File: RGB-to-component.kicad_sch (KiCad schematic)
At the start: 58 parts, among them J1 VGA, J3 USB_C_Receptacle_Power, J4 SCART_CONN, J5 3xRCA_CONN, U1 SC6206B-65K5, U10 74HC86, U3 RS8752XK, U6 THS7374, U8 LM1881

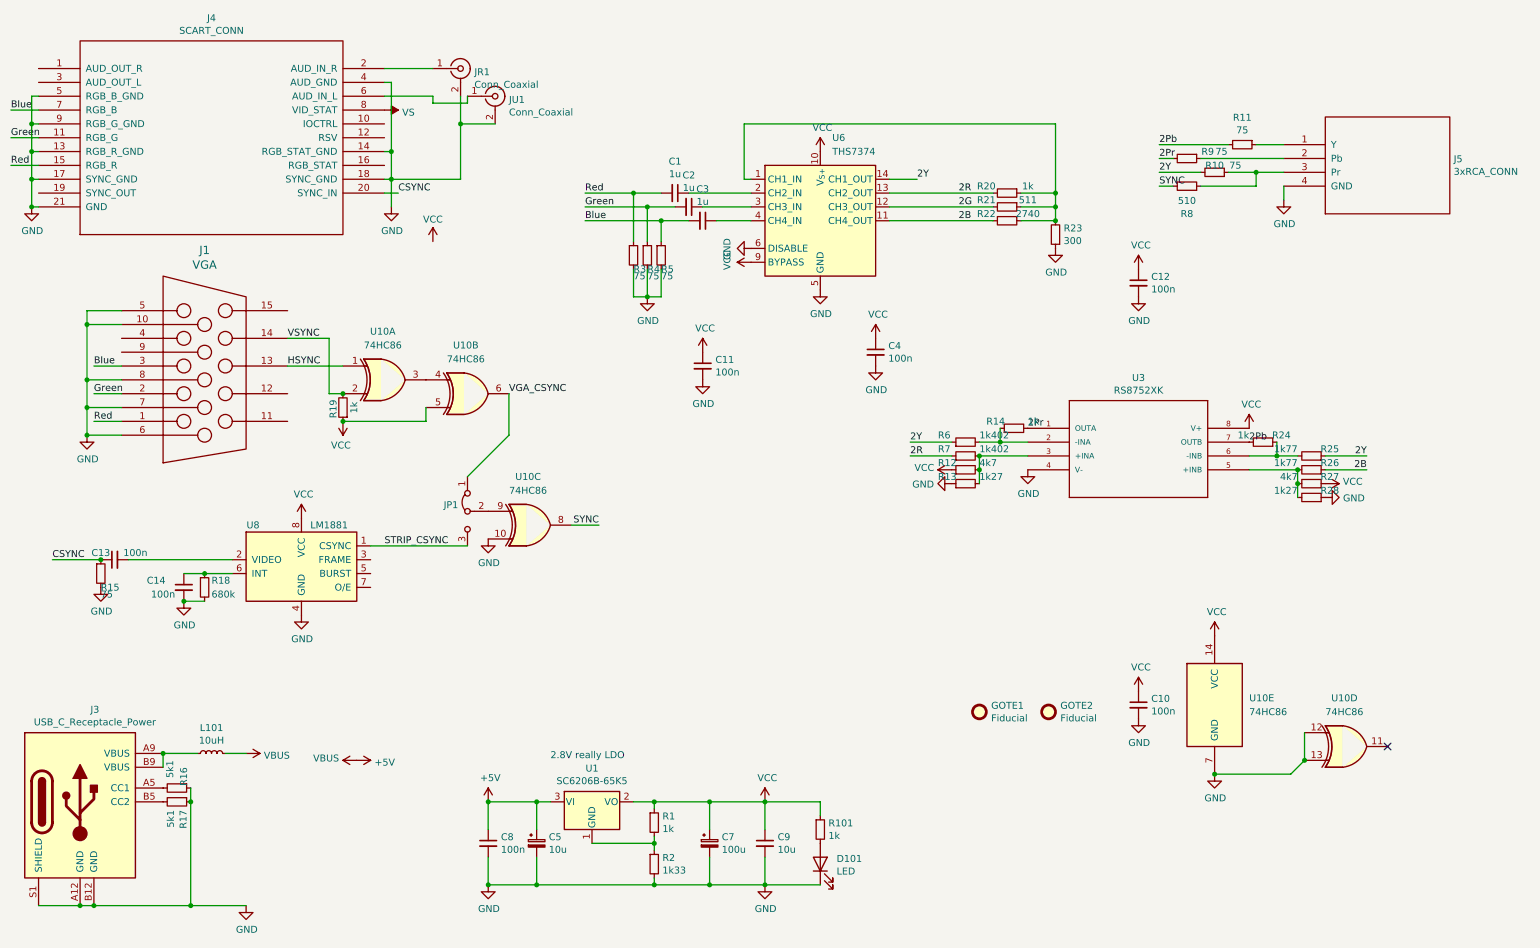
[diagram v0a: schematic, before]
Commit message: updated prod files
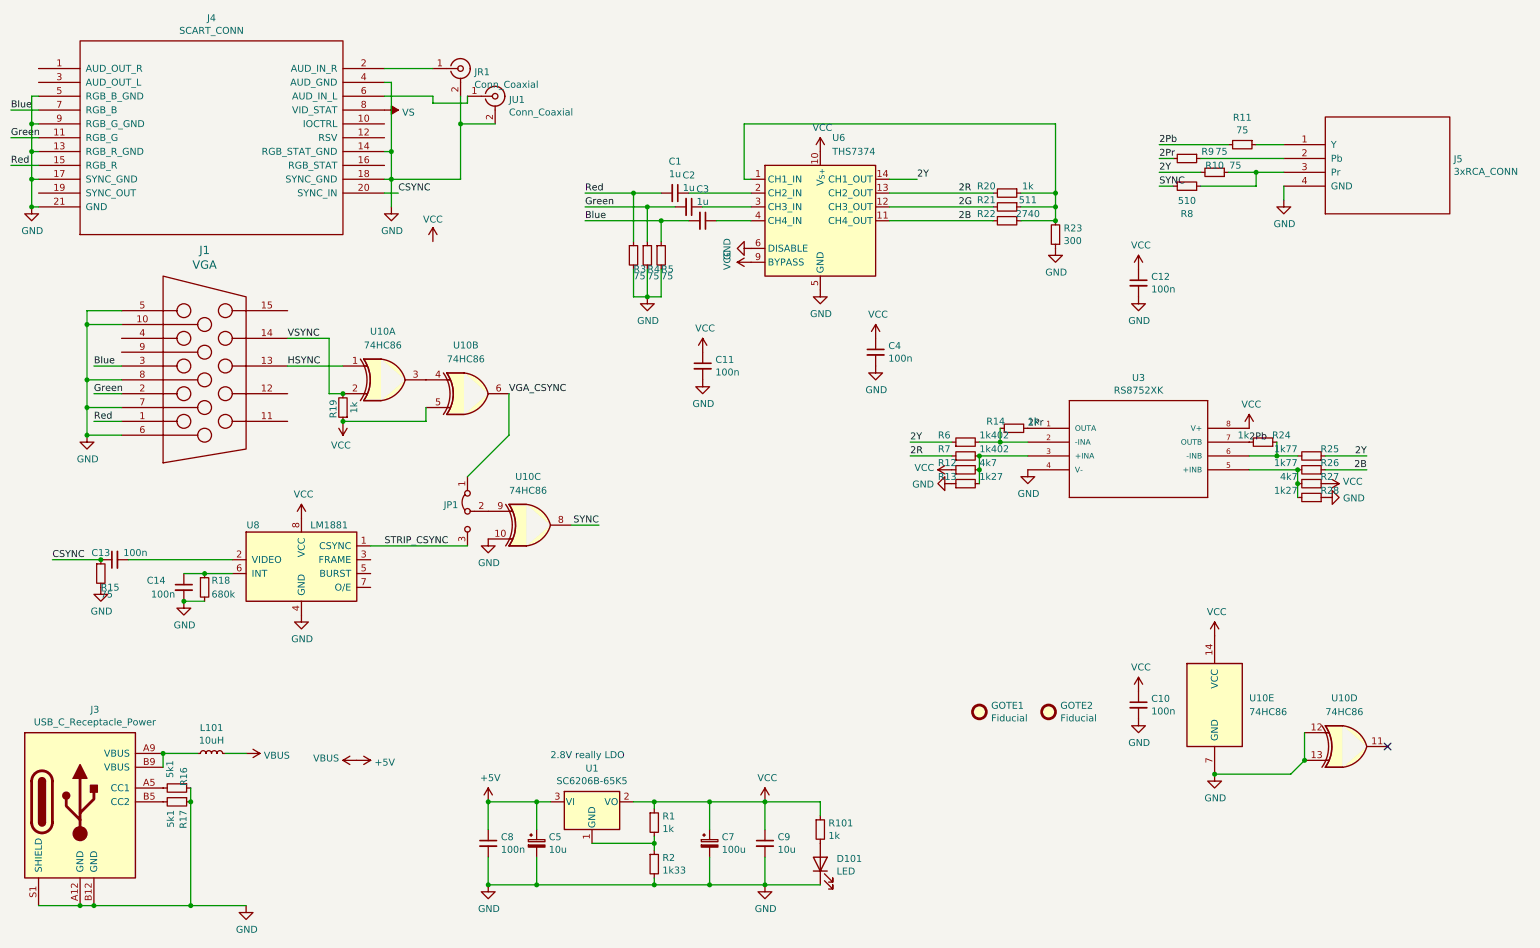
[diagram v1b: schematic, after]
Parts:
- U1: LCSC C130827 -> C2688243
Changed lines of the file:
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@@
 (kicad_sch
-	(version 20231120)
+	(version 20250114)
 	(generator "eeschema")
-	(generator_version "8.0")
+	(generator_version "9.0")
 	(paper "A4")
 	(title_block
@@
 		(comment 1 "KiCad gaming")
 	)
+	(text "2.8V really LDO"
+		(exclude_from_sim no)
+		(at 114.3 152.4 0)
+		(effects
+			(font
+				(size 1.27 1.27)
+			)
+			(justify left bottom)
+		)
+	)
 	(junction
 		(at 193.04 96.52)
@@
 		)
 	)
-	(text "2.8V really LDO"
-		(exclude_from_sim no)
-		(at 114.3 152.4 0)
-		(effects
-			(font
-				(size 1.27 1.27)
-			)
-			(justify left bottom)
-		)
-	)
 	(label "VGA_CSYNC"
 		(at 106.68 85.09 0)
-		(fields_autoplaced yes)
 		(effects
 			(font
@@
 	(label "2B"
 		(at 264.16 99.06 180)
-		(fields_autoplaced yes)
 		(effects
 			(font
@@
 	(label "Green"
 		(at 30.48 85.09 0)
-		(fields_autoplaced yes)
 		(effects
 			(font
@@
 	(label "Blue"
 		(at 120.65 53.34 0)
-		(fields_autoplaced yes)
 		(effects
 			(font
@@
 	(label "2Pb"
 		(at 242.57 93.98 0)
-		(fields_autoplaced yes)
 		(effects
 			(font
@@
 	(label "2Y"
 		(at 180.34 93.98 0)
-		(fields_autoplaced yes)
 		(effects
 			(font
@@
 	(label "Blue"
 		(at 15.24 33.02 0)
-		(fields_autoplaced yes)
 		(effects
 			(font
@@
 	(label "Green"
 		(at 120.65 50.8 0)
-		(fields_autoplaced yes)
 		(effects
 			(font
@@
 	(label "2G"
 		(at 189.23 50.8 0)
-		(fields_autoplaced yes)
 		(effects
 			(font
@@
 	(label "VSYNC"
 		(at 66.04 74.93 0)
-		(fields_autoplaced yes)
 		(effects
 			(font
@@
 	(label "2B"
 		(at 189.23 53.34 0)
-		(fields_autoplaced yes)
 		(effects
 			(font
@@
 	(label "CSYNC"
 		(at 86.36 48.26 0)
-		(fields_autoplaced yes)
 		(effects
 			(font
@@
 	(label "Red"
 		(at 30.48 90.17 0)
-		(fields_autoplaced yes)
 		(effects
 			(font
@@
 	(label "STRIP_CSYNC"
 		(at 83.82 113.03 0)
-		(fields_autoplaced yes)
 		(effects
 			(font
@@
 	(label "2Y"
 		(at 226.06 44.45 0)
-		(fields_autoplaced yes)
 		(effects
 			(font
@@
 	(label "2R"
 		(at 189.23 48.26 0)
-		(fields_autoplaced yes)
 		(effects
 			(font
@@
 	(label "2R"
 		(at 180.34 96.52 0)
-		(fields_autoplaced yes)
 		(effects
 			(font
@@
 	(label "Red"
 		(at 120.65 48.26 0)
-		(fields_autoplaced yes)
 		(effects
 			(font
@@
 	(label "2Y"
 		(at 264.16 96.52 180)
-		(fields_autoplaced yes)
 		(effects
 			(font
@@
 	(label "SYNC"
 		(at 226.06 46.99 0)
-		(fields_autoplaced yes)
 		(effects
 			(font
@@
 	(label "2Pr"
 		(at 201.93 91.44 0)
-		(fields_autoplaced yes)
 		(effects
 			(font
@@
 	(label "CSYNC"
 		(at 22.86 115.57 0)
-		(fields_autoplaced yes)
 		(effects
 			(font
@@
 	(label "2Y"
 		(at 181.61 45.72 0)
-		(fields_autoplaced yes)
 		(effects
 			(font
@@
 	(label "2Pb"
 		(at 226.06 39.37 0)
-		(fields_autoplaced yes)
 		(effects
 			(font
@@
 	(label "HSYNC"
 		(at 66.04 80.01 0)
-		(fields_autoplaced yes)
 		(effects
 			(font
@@
 	(label "2Pr"
 		(at 226.06 41.91 0)
-		(fields_autoplaced yes)
 		(effects
 			(font
@@
 	(label "Red"
 		(at 15.24 43.18 0)
-		(fields_autoplaced yes)
 		(effects
 			(font
@@
 	(label "Blue"
 		(at 30.48 80.01 0)
-		(fields_autoplaced yes)
 		(effects
 			(font
@@
 	(label "Green"
 		(at 15.24 38.1 0)
-		(fields_autoplaced yes)
 		(effects
 			(font
@@
 	(label "SYNC"
 		(at 123.19 109.22 180)
-		(fields_autoplaced yes)
 		(effects
 			(font
@@
 			)
 		)
-		(property "LCSC" "C130827"
+		(property "LCSC" "C2688243"
 			(at 121.92 160.02 0)
 			(effects
@@
 		)
 	)
+	(embedded_fonts no)
 )

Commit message: prod file update
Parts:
- R13, R28: LCSC C101451 -> C228375
- R2: LCSC C17382 -> C276298
- R25, R26: LCSC C17397 -> C706262
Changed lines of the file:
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@@
 			)
 		)
-		(property "LCSC" "C17382"
+		(property "LCSC" "C276298"
 			(at 133.35 171.45 0)
 			(effects
@@
 			)
 		)
-		(property "LCSC" "C101451"
+		(property "LCSC" "C228375"
 			(at 190.5 101.6 0)
 			(effects
@@
 			)
 		)
-		(property "LCSC" "C17397"
+		(property "LCSC" "C706262"
 			(at 254 99.06 0)
 			(effects
@@
 			)
 		)
-		(property "LCSC" "C101451"
+		(property "LCSC" "C228375"
 			(at 254 104.14 0)
 			(effects
@@
 			)
 		)
-		(property "LCSC" "C17397"
+		(property "LCSC" "C706262"
 			(at 254 96.52 0)
 			(effects

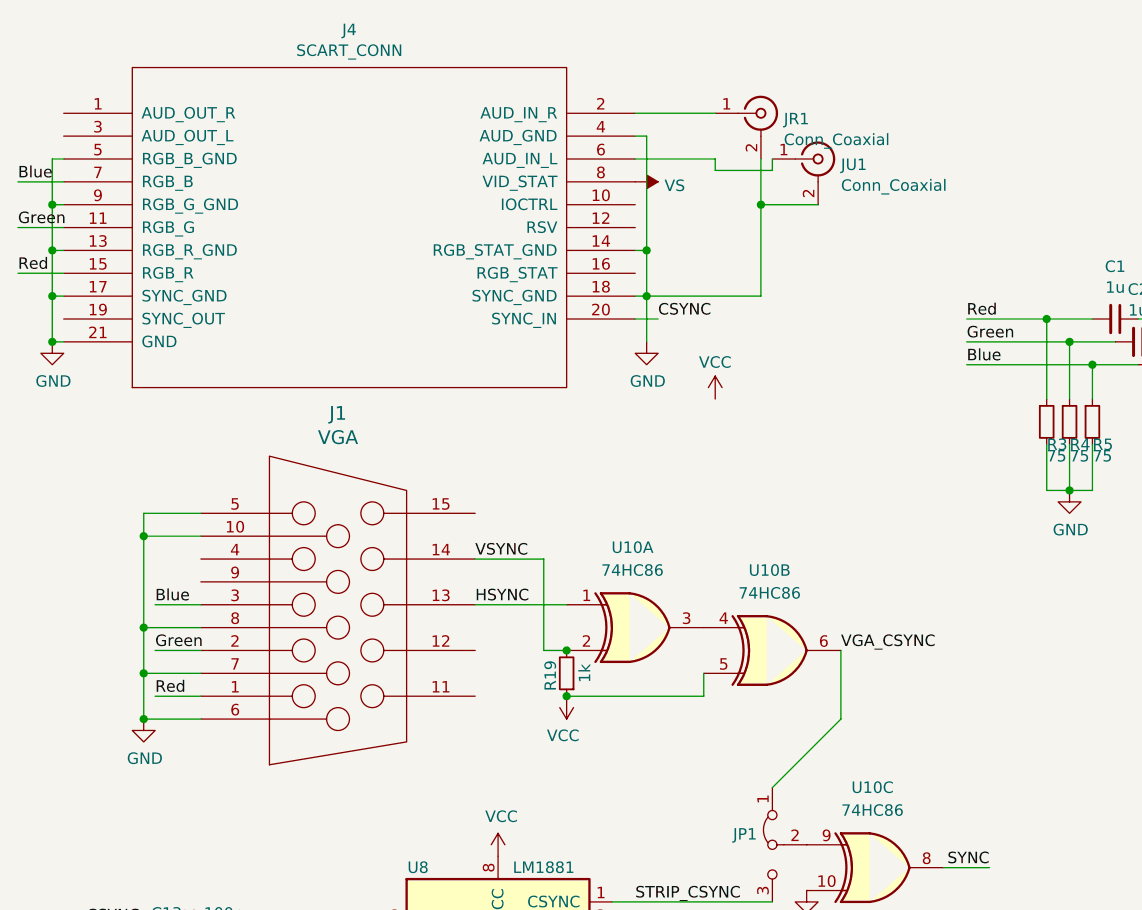
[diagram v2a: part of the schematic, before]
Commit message: .
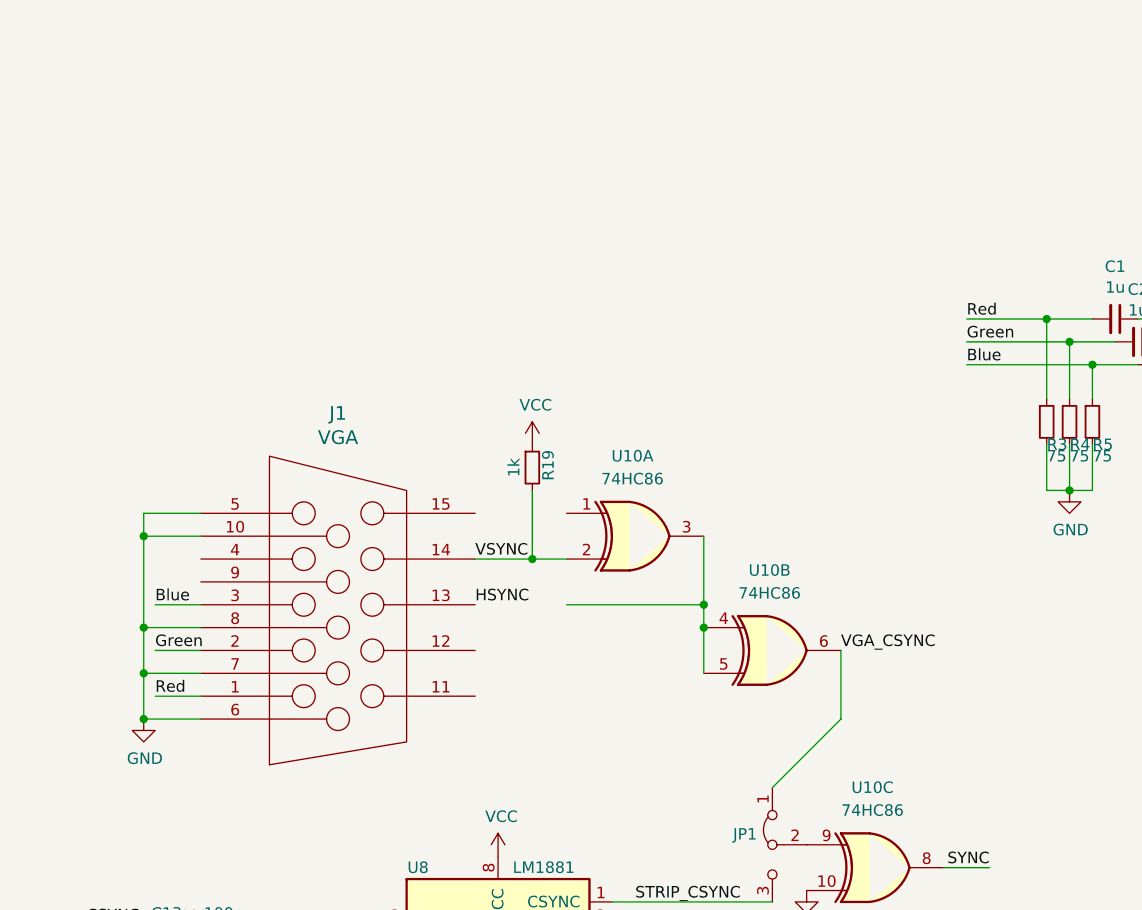
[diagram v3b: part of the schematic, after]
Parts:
- removed J4: SCART_CONN, custom_components:SCART_CONN, symbol RGB-to-component-rescue:SCART_CONN-ossc
- removed JR1, JU1: Conn_Coaxial, videobits:Cheapo_RCA_single_edge, symbol Connector:Conn_Coaxial
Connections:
- net HSYNC: no longer U10.1
- net VCC: no longer U10.5
- net at U10.3, U10.4: now also U10.5
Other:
- moved on the sheet: R19, U10A
